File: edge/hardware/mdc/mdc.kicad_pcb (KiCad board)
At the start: 2 copper layers, 117 x 122.5 mm, 35 parts, among them J1 IBT_2, J2 Screw_Terminal_01x02, J3 Screw_Terminal_01x02, J4 Screw_Terminal_01x02, Q1 2N7000, Q2 2N7000, Q3 2N7000, Q4 2N7000, U1 ESP32-S3-DEVKITC-1-N16R8V, U2 INMP441, U3 GY-906, U4 STEVAL-MKIGIBV2, U5 74HC04, U6 ACS712-30A

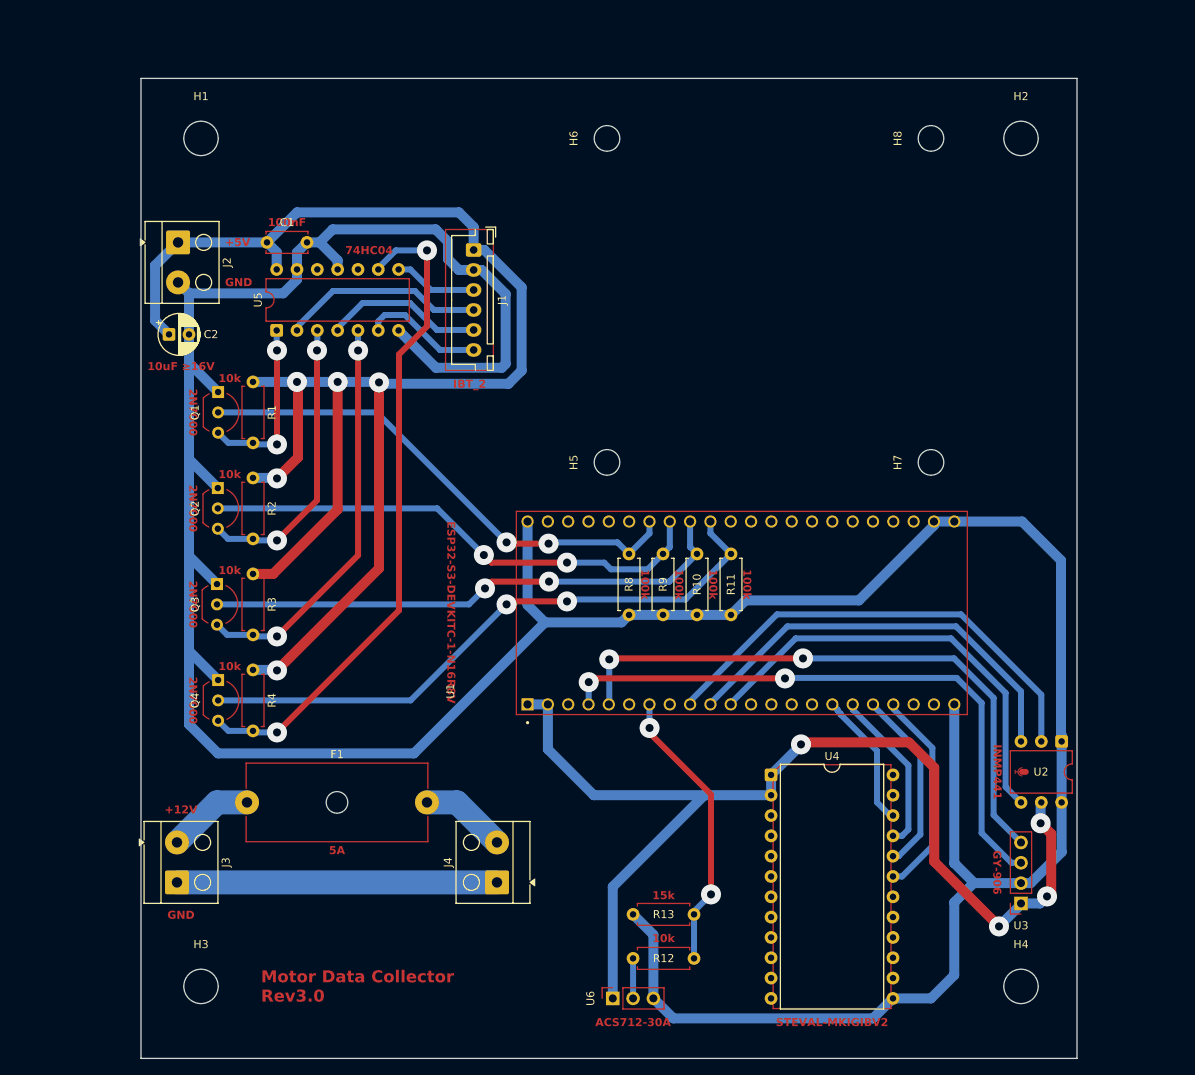
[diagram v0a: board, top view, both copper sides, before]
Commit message: update rev3.0 schematic and layout
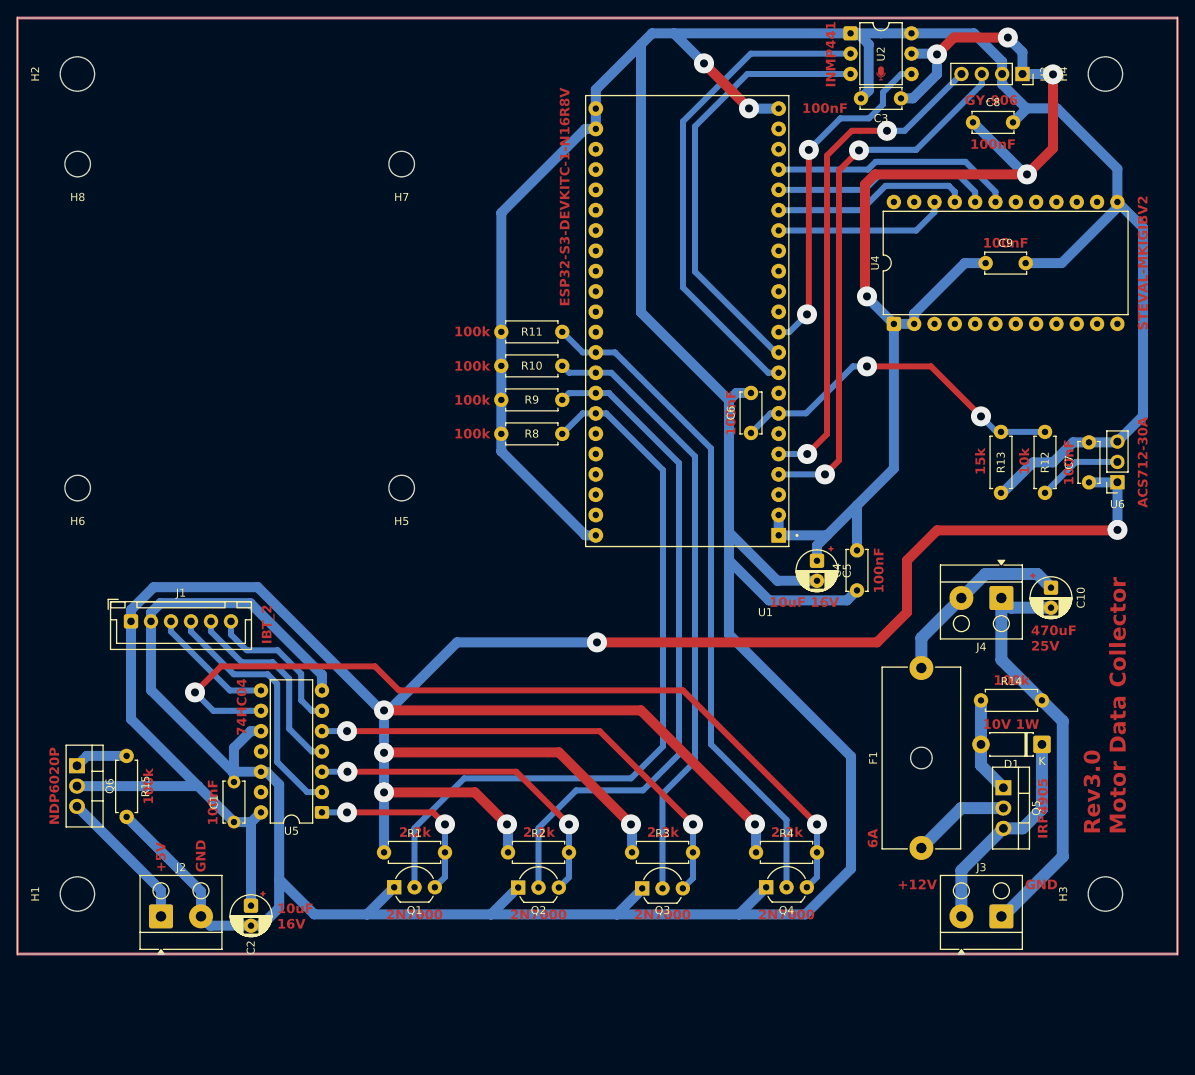
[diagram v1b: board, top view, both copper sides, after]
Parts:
- added C10: 470uF 25V, Capacitor_THT:CP_Radial_D5.0mm_P2.50mm, F.Cu at (197.5, 97.2)
- added C3: 100nF, Capacitor_THT:C_Disc_D5.0mm_W2.5mm_P5.00mm, F.Cu at (178.8, 36.0)
- added C4: 100nF, Capacitor_THT:C_Disc_D5.0mm_W2.5mm_P5.00mm, F.Cu at (173.2, 97.5)
- added C5: 10uF 16V, Capacitor_THT:CP_Radial_D5.0mm_P2.50mm, F.Cu at (168.2, 93.8)
- added C6: 100nF, Capacitor_THT:C_Disc_D5.0mm_W2.5mm_P5.00mm, F.Cu at (160.0, 77.8)
- added C7: 100nF, Capacitor_THT:C_Disc_D5.0mm_W2.5mm_P5.00mm, F.Cu at (202.2, 84.0)
- added C8: 100nF, Capacitor_THT:C_Disc_D5.0mm_W2.5mm_P5.00mm, F.Cu at (187.8, 39.0)
- added C9: 100nF, Capacitor_THT:C_Disc_D5.0mm_W2.5mm_P5.00mm, F.Cu at (189.3, 56.6)
- added D1: 10V 1W, Diode_THT:D_DO-41_SOD81_P7.62mm_Horizontal, F.Cu at (196.4, 116.8)
- added Q5: IRF4905, Package_TO_SOT_THT:TO-220-3_Vertical, F.Cu at (191.6, 122.2)
- added Q6: NDP6020P, Package_TO_SOT_THT:TO-220-3_Vertical, F.Cu at (75.8, 119.4)
- added R14: 100k, Resistor_THT:R_Axial_DIN0207_L6.3mm_D2.5mm_P7.62mm_Horizontal, F.Cu at (188.8, 111.2)
- added R15: 100k, Resistor_THT:R_Axial_DIN0207_L6.3mm_D2.5mm_P7.62mm_Horizontal, F.Cu at (82.0, 118.2)
- C2: value 10uF ≥16V -> 10uF 16V
- F1: value 5A -> 6A
- J1: value IBT_2 -> Conn_01x06
- R1, R2, R3, R4: value 10k -> 2.2k
- moved H2 118.2 mm to (75.8, 33.0), turned to 90 degrees
- moved H4 114.5 mm to (204.3, 33.0), turned to 90 degrees
- moved H3 113.6 mm to (204.3, 135.4), turned to 90 degrees
- moved H8 106.7 mm to (75.8, 44.2), turned to 180 degrees
- moved U3 103.7 mm to (193.9, 33.0), turned to -90 degrees
- moved J3 98.5 mm to (186.3, 138.2), turned to 0 degrees
- moved H1 95.7 mm to (75.8, 135.4), turned to 90 degrees
- moved U2 92.4 mm to (172.4, 27.9), turned to 0 degrees
- moved U6 90.2 mm to (205.8, 84.0), turned to 180 degrees
- moved F1 84.5 mm to (181.3, 129.7), turned to 90 degrees
- moved J2 84.3 mm to (86.2, 138.2), turned to 0 degrees
- moved H6 79.3 mm to (75.8, 84.7), turned to 180 degrees
- moved R12 77.7 mm to (196.8, 85.3), turned to 90 degrees
- moved H7 76.0 mm to (116.3, 44.2), turned to 180 degrees
- moved Q4 73.2 mm to (161.9, 134.6), turned to 0 degrees
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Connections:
- F1 pad 1: +12V -> Net-(Q5-D)
- J2 pad 1: +5V -> Net-(J2-Pin_1)
- U5 pad 10: unconnected-(U5-Pad10) -> GND
- U5 pad 11: GND -> unconnected-(U5-Pad11)
- U5 pad 12: unconnected-(U5-Pad12) -> GND
- U5 pad 13: GND -> unconnected-(U5-Pad13)
- U6 pad 1: +3V3 -> +5V
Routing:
- net GND: track 430.0 -> 596.2 mm, vias 0 -> 2
- net +5V: track 202.5 -> 347.2 mm, vias 5 -> 8
- net GPIO41: track 63.9 -> 93.8 mm, vias 2 -> 0
- net L_EN_IN: track 83.2 -> 104.9 mm
- net GPIO40: track 64.0 -> 83.8 mm, vias 2 -> 0
- net +3V3: track 137.9 -> 156.6 mm, vias 4 -> 5
- net Net-(J2-Pin_1): track 0.00 -> 18.1 mm
- net +12V: track 10.8 -> 27.1 mm
- net +12V_FUSED: track 10.8 -> 24.0 mm
- net MOTOR_GND: track 40.0 -> 53.1 mm
- net I2S_SD: track 55.2 -> 42.8 mm, vias 0 -> 2
- net I2C_SDA: track 75.3 -> 62.9 mm
- net Net-(Q5-D): track 0.00 -> 12.3 mm
- net Net-(D1-A): track 0.00 -> 12.1 mm
- net GPIO39: track 67.0 -> 77.0 mm, vias 2 -> 0
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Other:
- board size 117 x 122.5 mm -> 145 x 117 mm
- board text added: "10uF 16V"
- board text added: "470uF 25V"
- board text added: "IBT_2"
- board text added: "Rev3.0 Motor Data Collector"
- board text removed: "Motor Data Collector Rev3.0"
